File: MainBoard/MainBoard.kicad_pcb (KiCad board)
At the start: 2 copper layers, 31.8 x 110 mm, 41 parts, among them U1 TL074CN, U2 TL074CN, U3 TL074CN

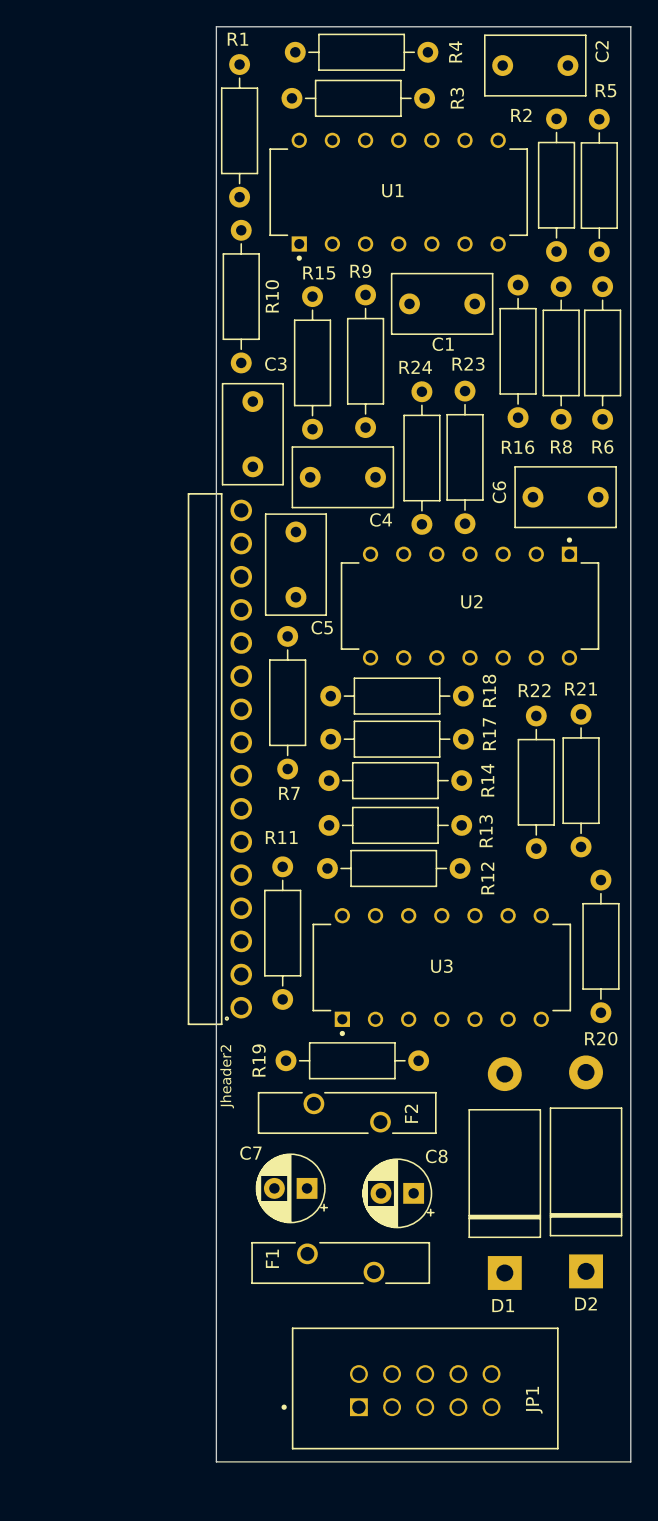
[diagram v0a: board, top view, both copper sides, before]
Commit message: updated placement
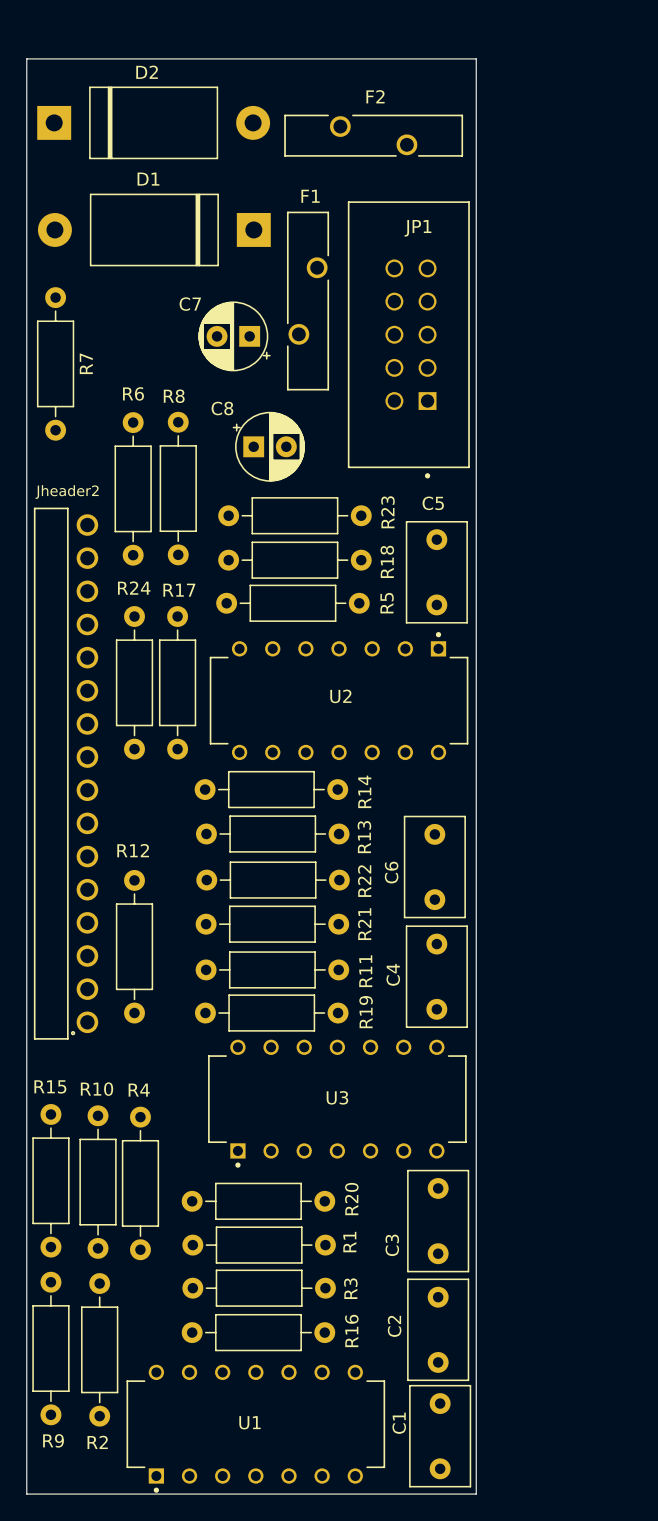
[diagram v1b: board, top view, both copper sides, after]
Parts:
- D1: value 1N5934B -> 1N5394B; footprint 1N5934B:P2_DO-201 -> 1N5349B:P2_DO-201
- D2: value 1N5934B -> 1N5349B; footprint 1N5934B:P2_DO-201 -> 1N5349B:P2_DO-201
- moved C2 99.5 mm to (169.3, 144.5), turned to 90 degrees
- moved U1 95.0 mm to (155.3, 149.3)
- moved R3 91.5 mm to (150.5, 138.8)
- moved R1 90.5 mm to (150.5, 135.5), turned to 0 degrees
- moved C1 89.3 mm to (169.4, 152.7), turned to 90 degrees
- moved R9 89.1 mm to (139.6, 148.5), turned to 90 degrees
- moved D2 86.9 mm to (147.5, 49.6), turned to 0 degrees
- moved R2 86.5 mm to (143.3, 138.5), turned to -90 degrees
- moved R4 82.4 mm to (146.5, 125.7), turned to -90 degrees
- moved R16 81.6 mm to (160.6, 142.2), turned to 180 degrees
- moved R10 78.8 mm to (143.2, 135.8), turned to 90 degrees
- moved JP1 77.3 mm to (168.5, 70.9), turned to 90 degrees
- moved D1 77.1 mm to (147.5, 57.8), turned to 180 degrees
- moved F2 74.9 mm to (164.3, 50.5), turned to 0 degrees
- moved F1 73.7 mm to (159.3, 63.2), turned to -90 degrees
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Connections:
- Jheader2 pad 12: Output8 -> Output5
- Jheader2 pad 13: Output9 -> Output8
- Jheader2 pad 14: Output10 -> Output6
- Jheader2 pad 7: Output5 -> Output9
- Jheader2 pad 8: Output6 -> Output10
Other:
- board size 31.8 x 110 mm -> 34.4 x 110 mm

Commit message: first pass at routing mainboard
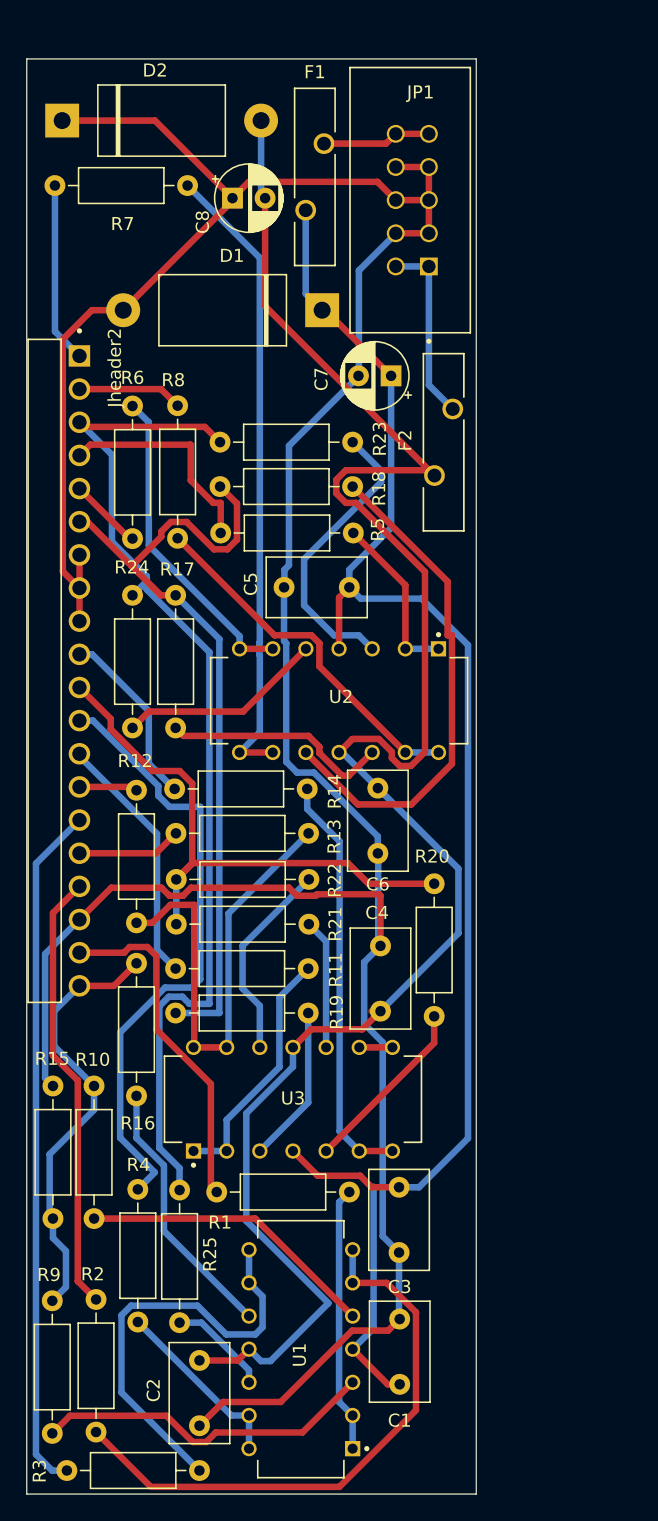
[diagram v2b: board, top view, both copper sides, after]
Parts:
- added R25: 100k, Resistor_THT:R_Axial_DIN0207_L6.3mm_D2.5mm_P10.16mm_Horizontal, F.Cu at (149.5, 141.5)
- Jheader2: footprint 61301611021:61301611021 -> 75168-116-20LF:AMPHENOL_75168-116-20LF
- moved F2 24.1 mm to (169.7, 74.0), turned to 90 degrees
- moved R16 23.2 mm to (146.2, 124.1), turned to 90 degrees
- moved C8 19.1 mm to (153.5, 55.3)
- moved R7 18.7 mm to (139.9, 54.4), turned to 0 degrees
- moved C2 18.3 mm to (151.0, 144.4), turned to -90 degrees
- moved R3 17.0 mm to (140.8, 152.8)
- moved R20 16.5 mm to (169.0, 118.0), turned to 90 degrees
- moved C7 11.2 mm to (165.7, 68.9)
- moved JP1 10.3 mm to (168.6, 60.6)
- moved F1 9.52 mm to (159.8, 53.7), turned to 90 degrees
- moved D1 8.07 mm to (152.8, 63.9)
- moved Jheader2 7.90 mm to (141.8, 91.5)
- moved C1 7.18 mm to (166.3, 146.2)
- moved R12 6.91 mm to (146.2, 100.7)
- moved C5 6.84 mm to (162.5, 85.1), turned to 180 degrees
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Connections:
- Jheader2 pad 10: InputBus4 -> Output10
- Jheader2 pad 11: Output7 -> InputBus4
- Jheader2 pad 12: Output5 -> Output4
- Jheader2 pad 13: Output8 -> Output9
- Jheader2 pad 14: Output6 -> Output12
- Jheader2 pad 15: Output11 -> Output3
- Jheader2 pad 16: Output12 -> Output11
- U1 pad 12: InputBus2 -> Net-(U1-4IN+)
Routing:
- net GND: track 0.00 -> 238.2 mm
- net -v: track 0.00 -> 144.6 mm
- net +v: track 0.00 -> 120.8 mm
- net InputBus2: track 0.00 -> 81.1 mm
- net InputBus3: track 0.00 -> 61.9 mm
- net Output3: track 0.00 -> 52.9 mm
- net Net-(U2-3IN-): track 0.00 -> 48.9 mm
- net Output4: track 0.00 -> 47.1 mm
- net Net-(U1-2IN-): track 0.00 -> 44.5 mm
- net InputBus4: track 0.00 -> 44.4 mm
- net Net-(U2-3IN+): track 0.00 -> 38.7 mm
- net Net-(U3-4IN-): track 0.00 -> 37.5 mm
- net Output2: track 0.00 -> 33.9 mm
- net InputBus1: track 0.00 -> 33.6 mm
- net Net-(U1-3IN-): track 0.00 -> 33.0 mm
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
